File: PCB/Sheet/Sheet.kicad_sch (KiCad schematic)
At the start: 9 parts, among them U1 ATtiny85-20S, U2 MAX3485, U3 ATtiny1616-M, U5 MCP9700Ax-ETT

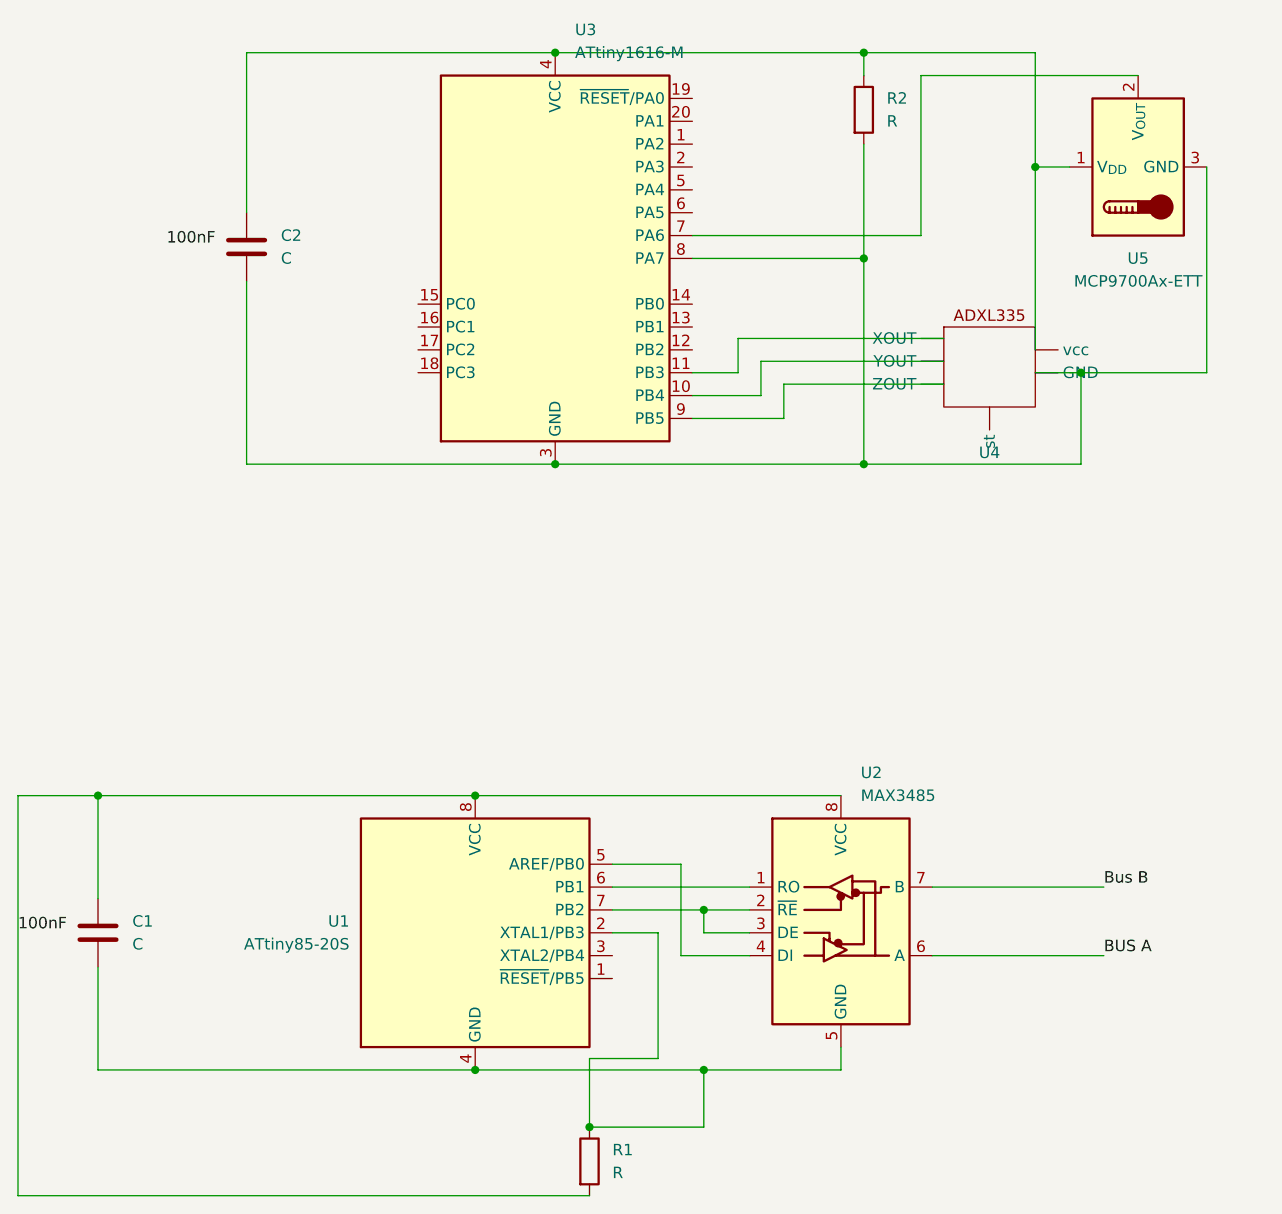
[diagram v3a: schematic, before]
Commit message: designs
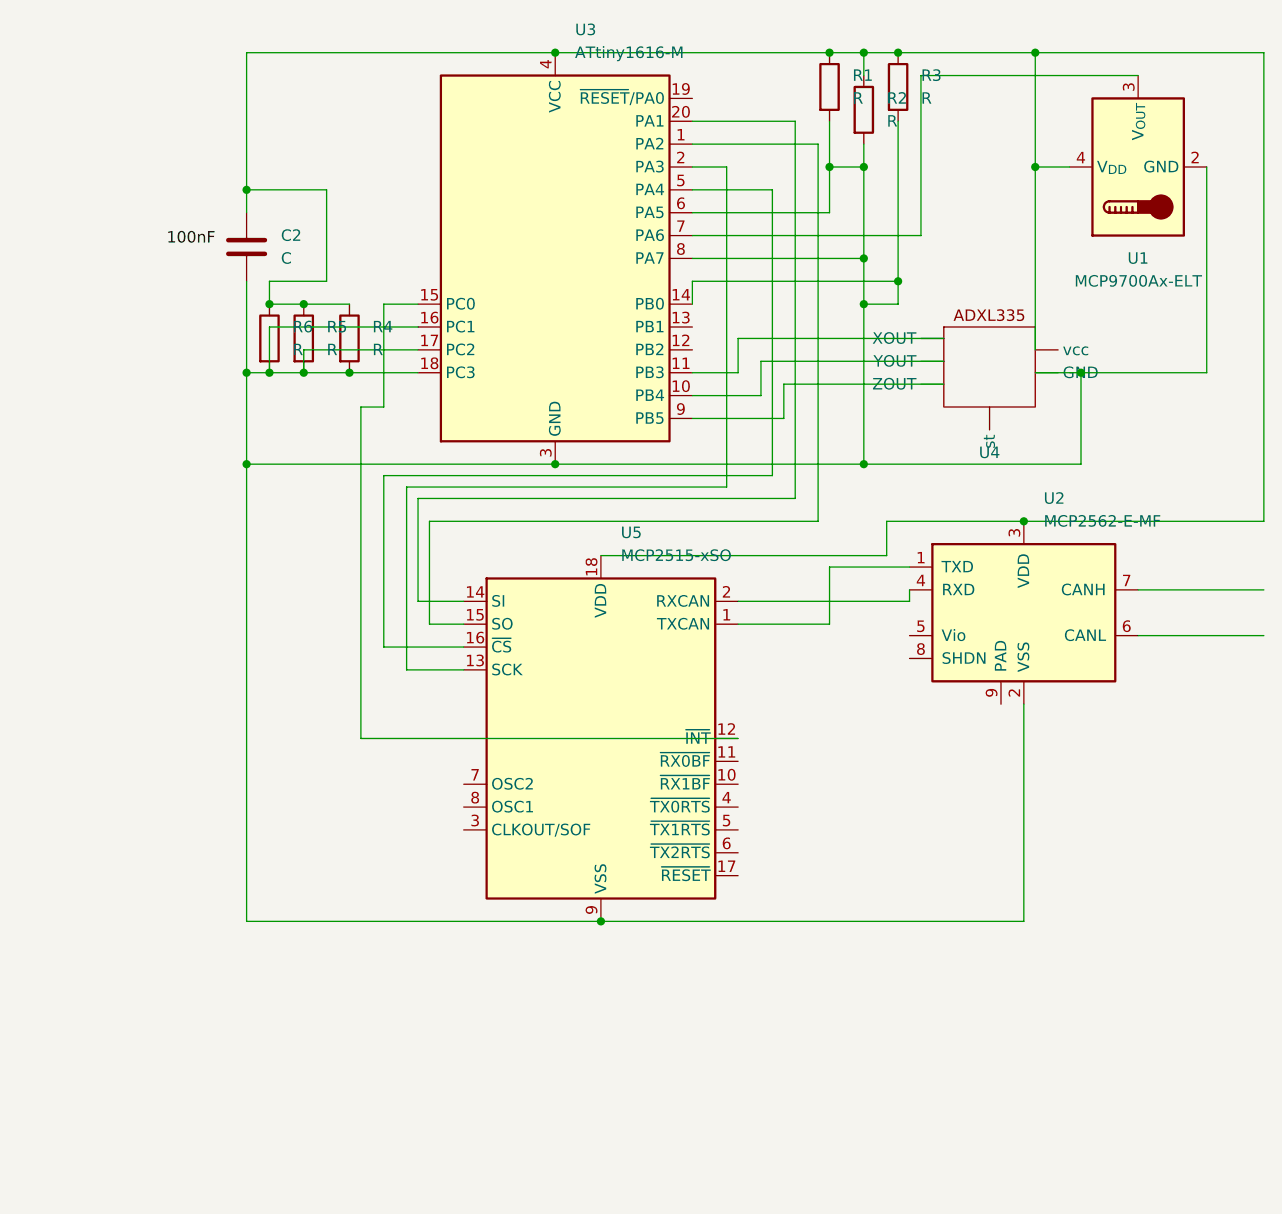
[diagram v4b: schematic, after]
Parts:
- removed C1: C, symbol Device:C
- removed U1: ATtiny85-20S, Package_SO:SOIC-8W_5.3x5.3mm_P1.27mm, symbol MCU_Microchip_ATtiny:ATtiny85-20S
- removed U2: MAX3485, symbol Interface_UART:MAX3485
- removed U5: MCP9700Ax-ETT, Package_TO_SOT_SMD:SOT-23, symbol Sensor_Temperature:MCP9700Ax-ETT
- added R3, R4, R5, R6: R, symbol Device:R
- added U1: MCP9700Ax-ELT, Package_TO_SOT_SMD:SOT-353_SC-70-5, symbol Sensor_Temperature:MCP9700Ax-ELT
- added U2: MCP2562-E-MF, Package_DFN_QFN:DFN-8-1EP_3x3mm_P0.65mm_EP1.55x2.4mm, symbol Interface_CAN_LIN:MCP2562-E-MF
- added U5: MCP2515-xSO, Package_SO:SOIC-18W_7.5x11.6mm_P1.27mm, symbol Interface_CAN_LIN:MCP2515-xSO
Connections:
- net 100nF: no longer R1.2
- net at R1.1: now also C2.1, R2.1, U3.4 (VCC), U4. (vcc), R3.1, R4.1, R5.1, R6.1, U1.4 (V_{DD}), U2.3 (VDD), U5.18 (VDD)
- net at U3.1 (PA2): now also U5.15 (SO)
- net at U3.14 (PB0): now also C2.2, R1.2, R2.2, U3.16 (PC1), U3.17 (PC2), U3.18 (PC3), U3.21 (GND), U3.3 (GND), U3.6 (PA5), U3.8 (PA7), U4. (vcc), R3.2, R4.2, R5.2, R6.2, U1.2 (GND), U2.2 (VSS), U5.9 (VSS)
- net at U3.15 (PC0): now also U5.12 (~{INT})
- net at U3.2 (PA3): now also U5.13 (SCK)
- net at U3.20 (PA1): now also U5.14 (SI)
- net at U3.5 (PA4): now also U5.16 (~{CS})
- net at U3.7 (PA6): now also U1.3 (V_{OUT})
- new net: U2.1 (TXD), U5.1 (TXCAN)
- new net: U2.4 (RXD), U5.2 (RXCAN)
- now unconnected: U4. (vcc), U4. (vcc)

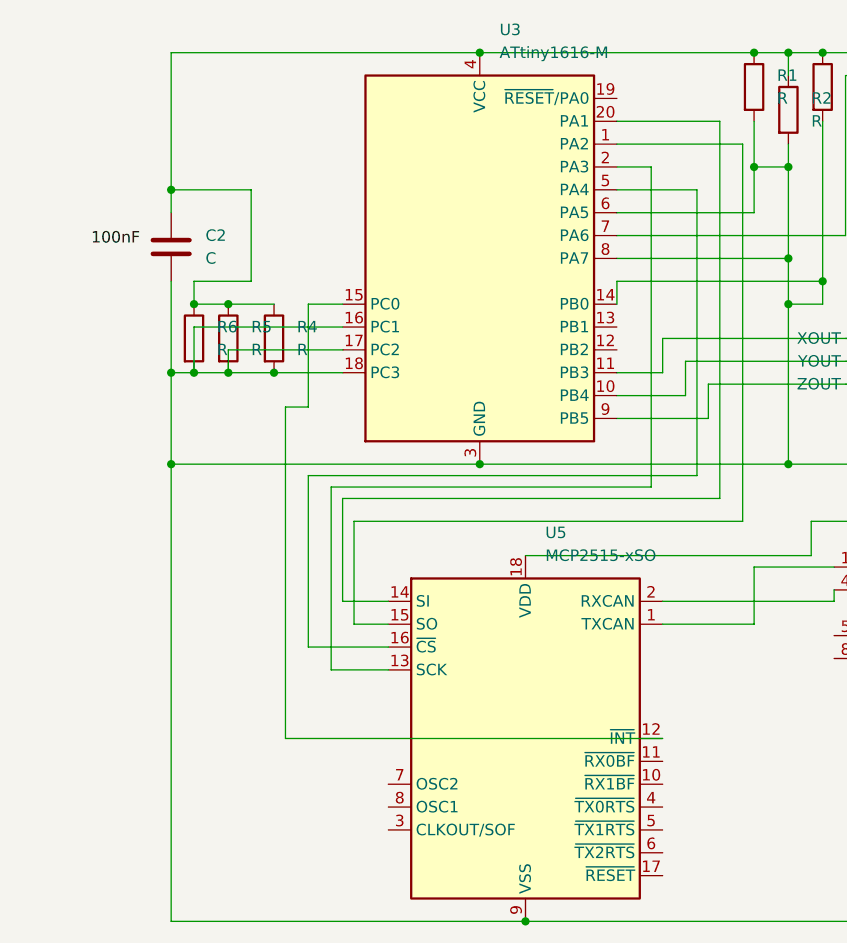
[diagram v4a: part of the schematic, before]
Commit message: PCB design
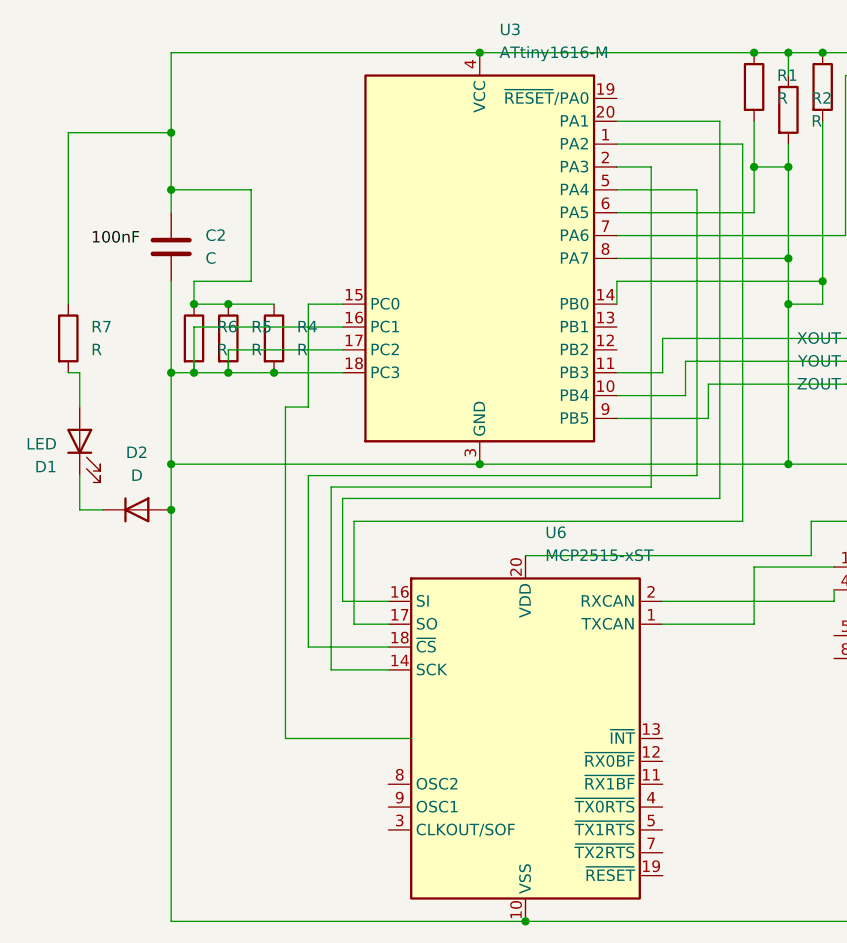
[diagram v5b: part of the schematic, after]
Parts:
- removed U5: MCP2515-xSO, Package_SO:SOIC-18W_7.5x11.6mm_P1.27mm, symbol Interface_CAN_LIN:MCP2515-xSO
- added D1: LED, symbol Device:LED
- added D2: D, symbol Device:D
- added R7: R, symbol Device:R
- added U6: MCP2515-xST, Package_SO:TSSOP-20_4.4x6.5mm_P0.65mm, symbol Interface_CAN_LIN:MCP2515-xST
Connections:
- net at C2.2, R1.2, R2.2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: now also D2.2 (A), U6.10 (VSS)
- net at C2.1, R1.1, R2.1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: now also R7.1, U6.20 (VDD)
- net at U3.1 (PA2): now also U6.17 (SO)
- net at U3.15 (PC0): now also U6.6 (NC)
- net at U3.2 (PA3): now also U6.14 (SCK)
- net at U3.20 (PA1): now also U6.16 (SI)
- net at U3.5 (PA4): now also U6.18 (~{CS})
- net at U2.1 (TXD): now also U6.1 (TXCAN)
- net at U2.4 (RXD): now also U6.2 (RXCAN)
- new net: D1.1 (K), D2.1 (K)
- new net: D1.2 (A), R7.2
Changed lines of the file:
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@@
   (junction (at 166.37 71.12) (diameter 0) (color 0 0 0 0)
   )
+  (junction (at 80.01 69.85) (diameter 0) (color 0 0 0 0)
+  )
   (junction (at 80.01 34.29) (diameter 0) (color 0 0 0 0)
   )
@@
   (junction (at 80.01 64.77) (diameter 0) (color 0 0 0 0)
   )
+  (junction (at 148.59 46.99) (diameter 0) (color 0 0 0 0)
+  )
   (junction (at 119.38 115.57) (diameter 0) (color 0 0 0 0)
   )
-  (junction (at 148.59 46.99) (diameter 0) (color 0 0 0 0)
-  )
   (junction (at 148.59 19.05) (diameter 0) (color 0 0 0 0)
   )
@@
   (junction (at 144.78 19.05) (diameter 0) (color 0 0 0 0)
   )
+  (junction (at 80.01 27.94) (diameter 0) (color 0 0 0 0)
+  )
   (junction (at 148.59 41.91) (diameter 0) (color 0 0 0 0)
   )
@@
   (junction (at 114.3 19.05) (diameter 0) (color 0 0 0 0)
   )
+  (wire (pts (xy 80.01 69.85) (xy 80.01 64.77))
+    (stroke (width 0) (type default))
+  )
   (wire (pts (xy 82.55 46.99) (xy 82.55 44.45))
     (stroke (width 0) (type default))
@@
     (stroke (width 0) (type default))
   )
+  (wire (pts (xy 69.85 54.61) (xy 69.85 58.42))
+    (stroke (width 0) (type default))
+  )
   (wire (pts (xy 86.36 46.99) (xy 91.44 46.99))
     (stroke (width 0) (type default))
   )
+  (wire (pts (xy 106.68 95.25) (xy 92.71 95.25))
+    (stroke (width 0) (type default))
+  )
   (wire (pts (xy 148.59 21.59) (xy 148.59 19.05))
     (stroke (width 0) (type default))
@@
     (stroke (width 0) (type default))
   )
-  (wire (pts (xy 134.62 95.25) (xy 92.71 95.25))
-    (stroke (width 0) (type default))
-  )
   (wire (pts (xy 82.55 46.99) (xy 86.36 46.99))
     (stroke (width 0) (type default))
@@
     (stroke (width 0) (type default))
   )
+  (wire (pts (xy 69.85 66.04) (xy 69.85 69.85))
+    (stroke (width 0) (type default))
+  )
   (wire (pts (xy 167.64 31.75) (xy 171.45 31.75))
     (stroke (width 0) (type default))
@@
     (stroke (width 0) (type default))
   )
+  (wire (pts (xy 119.38 115.57) (xy 166.37 115.57))
+    (stroke (width 0) (type default))
+  )
+  (wire (pts (xy 68.58 27.94) (xy 80.01 27.94))
+    (stroke (width 0) (type default))
+  )
   (wire (pts (xy 99.06 52.07) (xy 86.36 52.07))
     (stroke (width 0) (type default))
@@
     (stroke (width 0) (type default))
   )
-  (wire (pts (xy 119.38 115.57) (xy 166.37 115.57))
+  (wire (pts (xy 80.01 115.57) (xy 119.38 115.57))
     (stroke (width 0) (type default))
   )
@@
     (stroke (width 0) (type default))
   )
-  (wire (pts (xy 80.01 115.57) (xy 80.01 64.77))
+  (wire (pts (xy 80.01 69.85) (xy 80.01 115.57))
     (stroke (width 0) (type default))
   )
@@
     (stroke (width 0) (type default))
   )
+  (wire (pts (xy 80.01 27.94) (xy 80.01 34.29))
+    (stroke (width 0) (type default))
+  )
   (wire (pts (xy 133.35 31.75) (xy 133.35 67.31))
     (stroke (width 0) (type default))
   )
+  (wire (pts (xy 68.58 54.61) (xy 69.85 54.61))
+    (stroke (width 0) (type default))
+  )
   (wire (pts (xy 100.33 71.12) (xy 100.33 82.55))
     (stroke (width 0) (type default))
@@
     (stroke (width 0) (type default))
   )
+  (wire (pts (xy 72.39 69.85) (xy 69.85 69.85))
+    (stroke (width 0) (type default))
+  )
   (wire (pts (xy 129.54 31.75) (xy 133.35 31.75))
     (stroke (width 0) (type default))
@@
     (stroke (width 0) (type default))
   )
-  (wire (pts (xy 119.38 115.57) (xy 80.01 115.57))
+  (wire (pts (xy 68.58 46.99) (xy 68.58 27.94))
     (stroke (width 0) (type default))
   )
@@
     (stroke (width 0) (type default))
   )
-  (wire (pts (xy 80.01 19.05) (xy 80.01 34.29))
+  (wire (pts (xy 80.01 19.05) (xy 80.01 27.94))
     (stroke (width 0) (type default))
   )
@@
     )
   )
+  (symbol (lib_id "Interface_CAN_LIN:MCP2515-xST") (at 119.38 95.25 0) (unit 1)
+    (in_bom yes) (on_board yes) (dnp no) (fields_autoplaced)
+    (property "Reference" "U6" (at 121.5741 72.39 0)
+      (effects (font (size 1.27 1.27)) (justify left))
+    )
+    (property "Value" "MCP2515-xST" (at 121.5741 74.93 0)
+      (effects (font (size 1.27 1.27)) (justify left))
+    )
+    (property "Footprint" "Package_SO:TSSOP-20_4.4x6.5mm_P0.65mm" (at 119.38 118.11 0)
+      (effects (font (size 1.27 1.27) italic) hide)
+    )
+    (property "Datasheet" "http://ww1.microchip.com/downloads/en/DeviceDoc/21801e.pdf" (at 121.92 115.57 0)
+      (effects (font (size 1.27 1.27)) hide)
+    )
+    (pin "8")
+    (pin "9")
+    (pin "2")
+    (pin "15")
+    (pin "14")
+    (pin "6")
+    (pin "19")
+    (pin "17")
+    (pin "7")
+    (pin "13")
+    (pin "12")
+    (pin "3")
+    (pin "11")
+    (pin "5")
+    (pin "1")
+    (pin "10")
+    (pin "18")
+    (pin "20")
+    (pin "16")
+    (pin "4")
+    (instances
+      (project "Sheet"
+        (path "/3799ba30-20d0-42d8-8664-7c6f9d1278f6"
+          (reference "U6") (unit 1)
+        )
+      )
+    )
+  )
   (symbol (lib_id "Device:R") (at 148.59 25.4 0) (unit 1)
     (in_bom yes) (on_board yes) (dnp no) (fields_autoplaced)
@@
     )
   )
+  (symbol (lib_id "Device:LED") (at 69.85 62.23 90) (unit 1)
+    (in_bom yes) (on_board yes) (dnp no)
+    (property "Reference" "D1" (at 67.31 65.0875 90)
+      (effects (font (size 1.27 1.27)) (justify left))
+    )
+    (property "Value" "LED" (at 67.31 62.5475 90)
+      (effects (font (size 1.27 1.27)) (justify left))
+    )
+    (property "Footprint" "" (at 69.85 62.23 0)
+      (effects (font (size 1.27 1.27)) hide)
+    )
+    (property "Datasheet" "~" (at 69.85 62.23 0)
+      (effects (font (size 1.27 1.27)) hide)
+    )
+    (pin "1")
+    (pin "2")
+    (instances
+      (project "Sheet"
+        (path "/3799ba30-20d0-42d8-8664-7c6f9d1278f6"
+          (reference "D1") (unit 1)
+        )
+      )
+    )
+  )
   (symbol (lib_id "Device:R") (at 91.44 50.8 0) (unit 1)
     (in_bom yes) (on_board yes) (dnp no) (fields_autoplaced)
@@
     )
   )
-  (symbol (lib_id "Interface_CAN_LIN:MCP2515-xSO") (at 119.38 95.25 0) (unit 1)
-    (in_bom yes) (on_board yes) (dnp no) (fields_autoplaced)
-    (property "Reference" "U5" (at 121.5741 72.39 0)
-      (effects (font (size 1.27 1.27)) (justify left))
-    )
-    (property "Value" "MCP2515-xSO" (at 121.5741 74.93 0)
-      (effects (font (size 1.27 1.27)) (justify left))
-    )
-    (property "Footprint" "Package_SO:SOIC-18W_7.5x11.6mm_P1.27mm" (at 119.38 118.11 0)
-      (effects (font (size 1.27 1.27) italic) hide)
-    )
-    (property "Datasheet" "http://ww1.microchip.com/downloads/en/DeviceDoc/21801e.pdf" (at 121.92 115.57 0)
-      (effects (font (size 1.27 1.27)) hide)
-    )
-    (pin "9")
-    (pin "12")
-    (pin "11")
-    (pin "4")
-    (pin "8")
-    (pin "5")
-    (pin "2")
-    (pin "17")
-    (pin "7")
-    (pin "18")
-    (pin "3")
-    (pin "16")
-    (pin "1")
-    (pin "14")
-    (pin "6")
-    (pin "10")
-    (pin "13")
-    (pin "15")
-    (instances
-      (project "Sheet"
-        (path "/3799ba30-20d0-42d8-8664-7c6f9d1278f6"
-          (reference "U5") (unit 1)
-        )
-      )
+  (symbol (lib_id "Device:R") (at 68.58 50.8 0) (unit 1)
+    (in_bom yes) (on_board yes) (dnp no) (fields_autoplaced)
+    (property "Reference" "R7" (at 71.12 49.53 0)
+      (effects (font (size 1.27 1.27)) (justify left))
+    )
+    (property "Value" "R" (at 71.12 52.07 0)
+      (effects (font (size 1.27 1.27)) (justify left))
+    )
+    (property "Footprint" "" (at 66.802 50.8 90)
+      (effects (font (size 1.27 1.27)) hide)
+    )
+    (property "Datasheet" "~" (at 68.58 50.8 0)
+      (effects (font (size 1.27 1.27)) hide)
+    )
+    (pin "1")
+    (pin "2")
+    (instances
+      (project "Sheet"
+        (path "/3799ba30-20d0-42d8-8664-7c6f9d1278f6"
+          (reference "R7") (unit 1)
+        )
+      )
+    )
+  )
+  (symbol (lib_id "Device:D") (at 76.2 69.85 0) (unit 1)
+    (in_bom yes) (on_board yes) (dnp no) (fields_autoplaced)
+    (property "Reference" "D2" (at 76.2 63.5 0)
+      (effects (font (size 1.27 1.27)))
+    )
+    (property "Value" "D" (at 76.2 66.04 0)
+      (effects (font (size 1.27 1.27)))
+    )
+    (property "Footprint" "" (at 76.2 69.85 0)
+      (effects (font (size 1.27 1.27)) hide)
+    )
+    (property "Datasheet" "~" (at 76.2 69.85 0)
+      (effects (font (size 1.27 1.27)) hide)
+    )
+    (property "Sim.Device" "D" (at 76.2 69.85 0)
+      (effects (font (size 1.27 1.27)) hide)
+    )
+    (property "Sim.Pins" "1=K 2=A" (at 76.2 69.85 0)
+      (effects (font (size 1.27 1.27)) hide)
+    )
+    (pin "1")
+    (pin "2")
+    (instances
+      (project "Sheet"
+        (path "/3799ba30-20d0-42d8-8664-7c6f9d1278f6"
+          (reference "D2") (unit 1)
+        )
+      )
